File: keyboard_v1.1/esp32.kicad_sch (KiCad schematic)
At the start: 9 parts, among them SW14 SW_DIP_x01, SW15 SW_DIP_x01, SW16 SW_DIP_x01, SW17 SW_DIP_x01

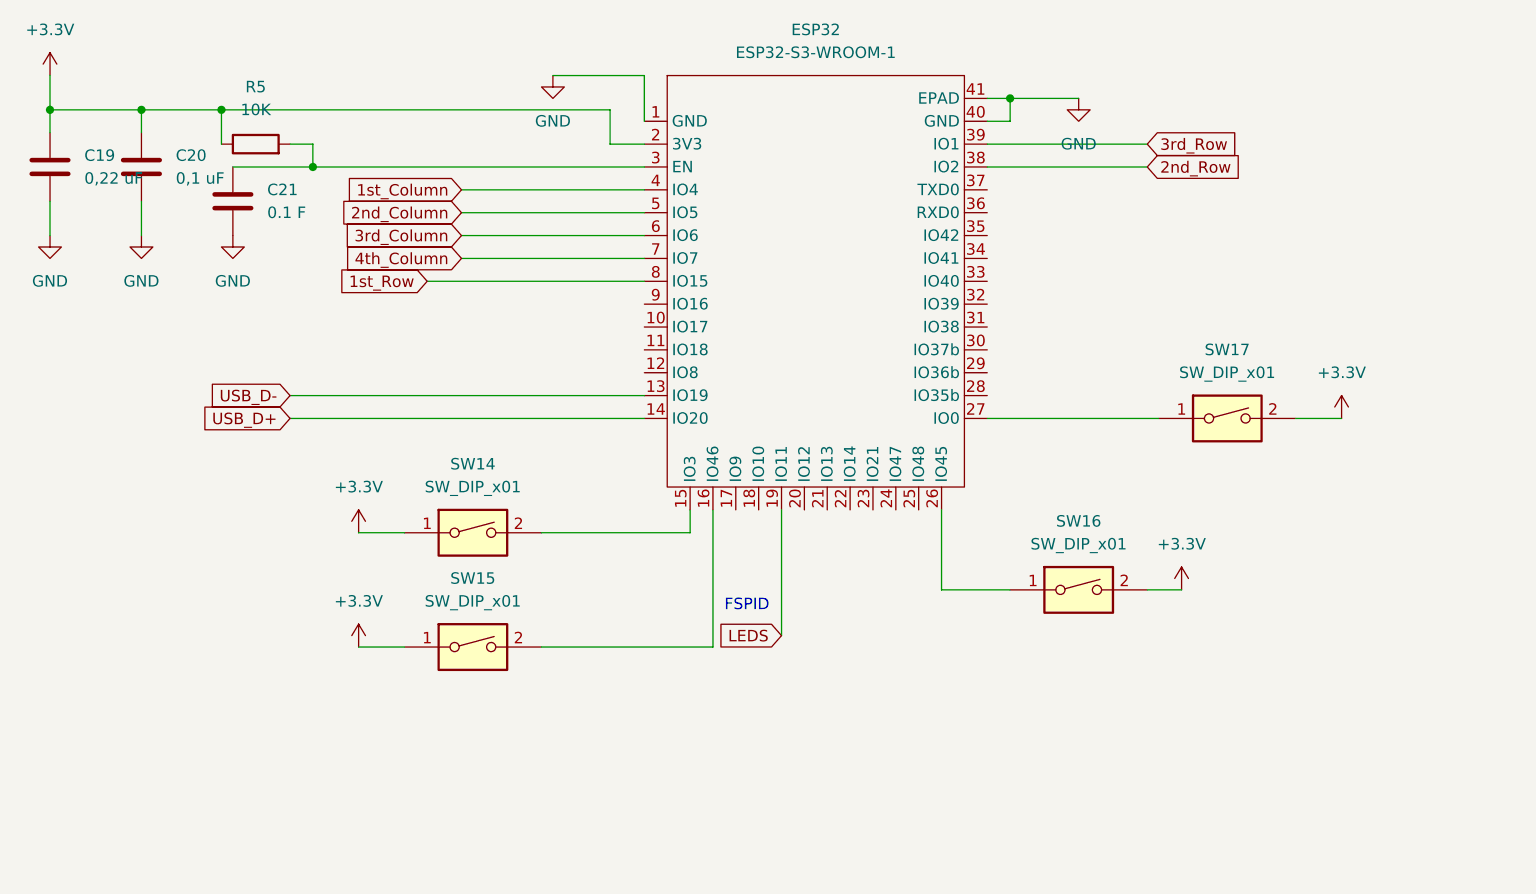
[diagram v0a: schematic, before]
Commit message: PCB layout done - 2022.07.25.
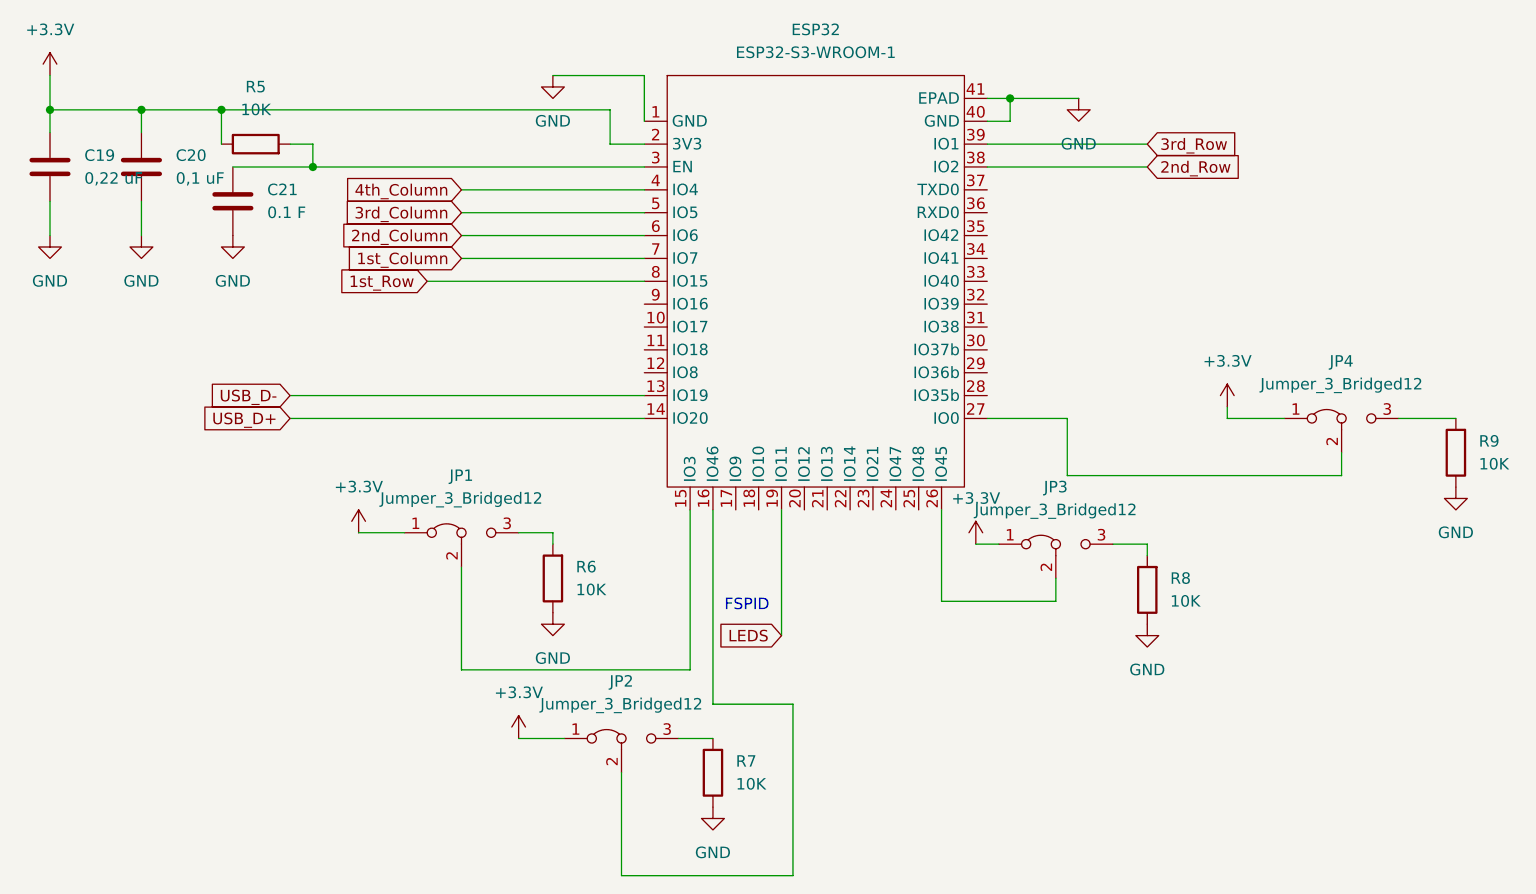
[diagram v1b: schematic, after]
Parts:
- removed SW14, SW15, SW16, SW17: SW_DIP_x01, Connector_PinHeader_2.54mm:PinHeader_1x02_P2.54mm_Vertical, symbol Switch:SW_DIP_x01
- added JP1, JP2, JP3, JP4: Jumper_3_Bridged12, Connector_PinHeader_2.54mm:PinHeader_1x03_P2.54mm_Horizontal, symbol Jumper:Jumper_3_Bridged12
- added R6, R7, R8, R9: 10K, Resistor_SMD:R_0805_2012Metric_Pad1.20x1.40mm_HandSolder, symbol Device:R
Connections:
- net +3V3: now also JP1.1 (A), JP2.1 (A), JP3.1 (A), JP4.1 (A)
- net 1st_Column: now also ESP32.7 (IO7); no longer ESP32.4 (IO4)
- net 2nd_Column: now also ESP32.6 (IO6); no longer ESP32.5 (IO5)
- net 3rd_Column: now also ESP32.5 (IO5); no longer ESP32.6 (IO6)
- net 4th_Column: now also ESP32.4 (IO4); no longer ESP32.7 (IO7)
- net GND: now also R6.1, R7.1, R8.1, R9.1
- net at ESP32.16 (IO46): now also JP2.2 (C)
- net at ESP32.15 (IO3): now also JP1.2 (C)
- net at ESP32.26 (IO45): now also JP3.2 (C)
- net at ESP32.27 (IO0): now also JP4.2 (C)
- new net: JP3.3 (B), R8.2
- new net: JP4.3 (B), R9.2
- new net: JP2.3 (B), R7.2
- new net: JP1.3 (B), R6.2
